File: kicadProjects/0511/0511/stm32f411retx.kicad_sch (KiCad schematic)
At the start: 9 parts, among them U8 STM32F411RETx

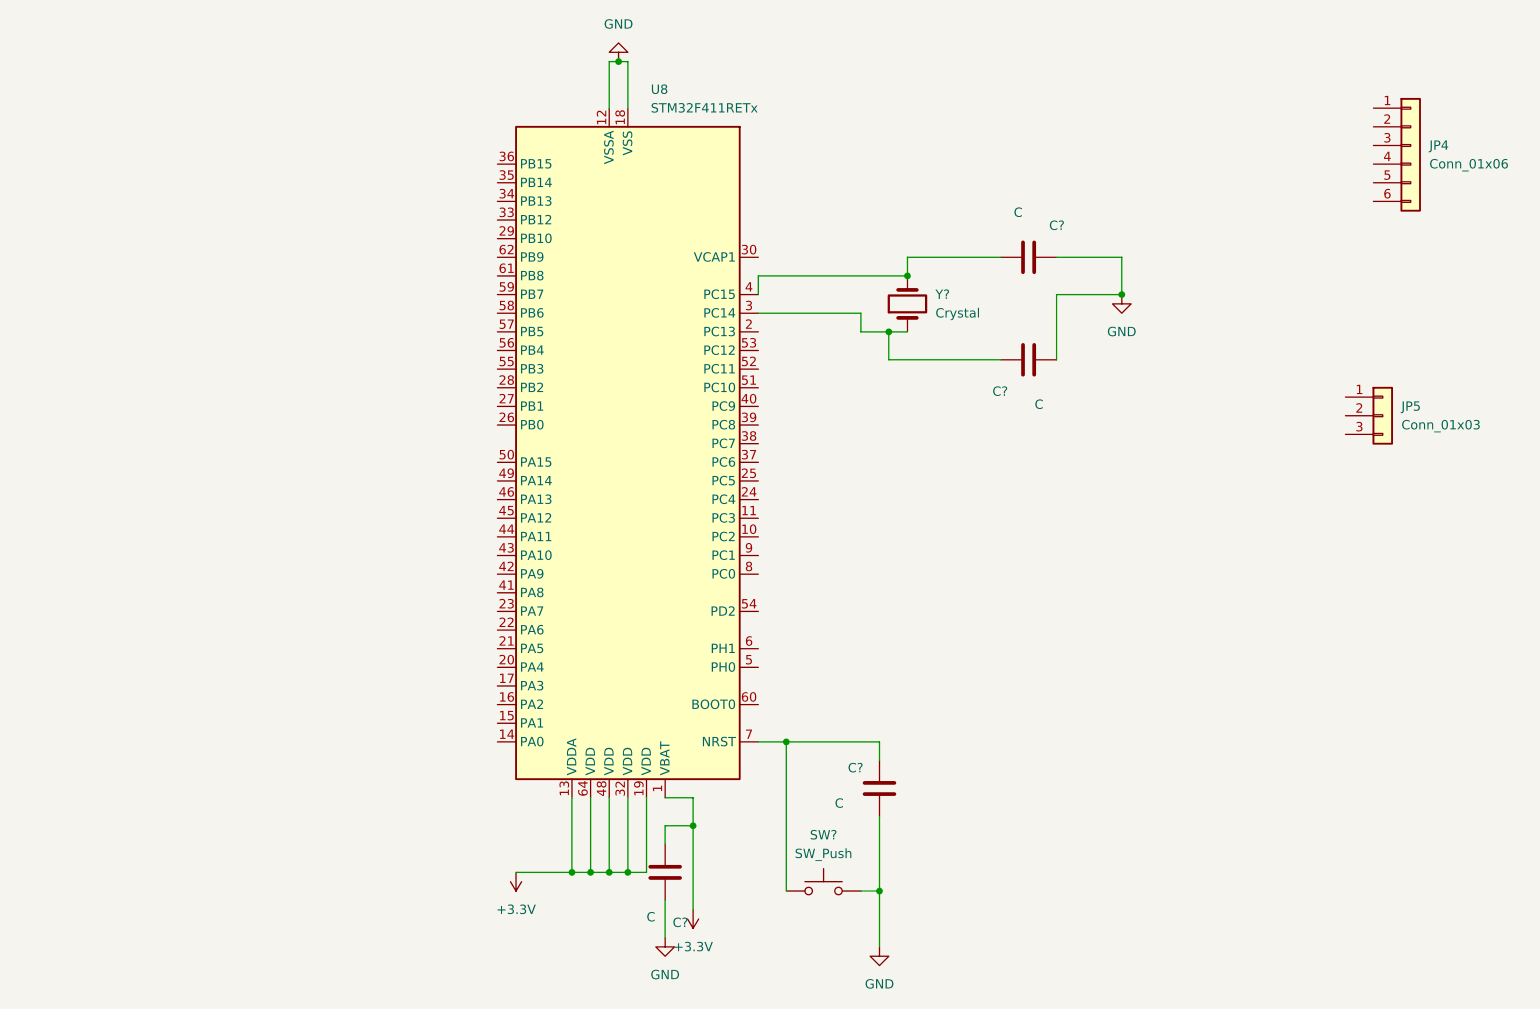
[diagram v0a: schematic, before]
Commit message: stm32 bloc implementation
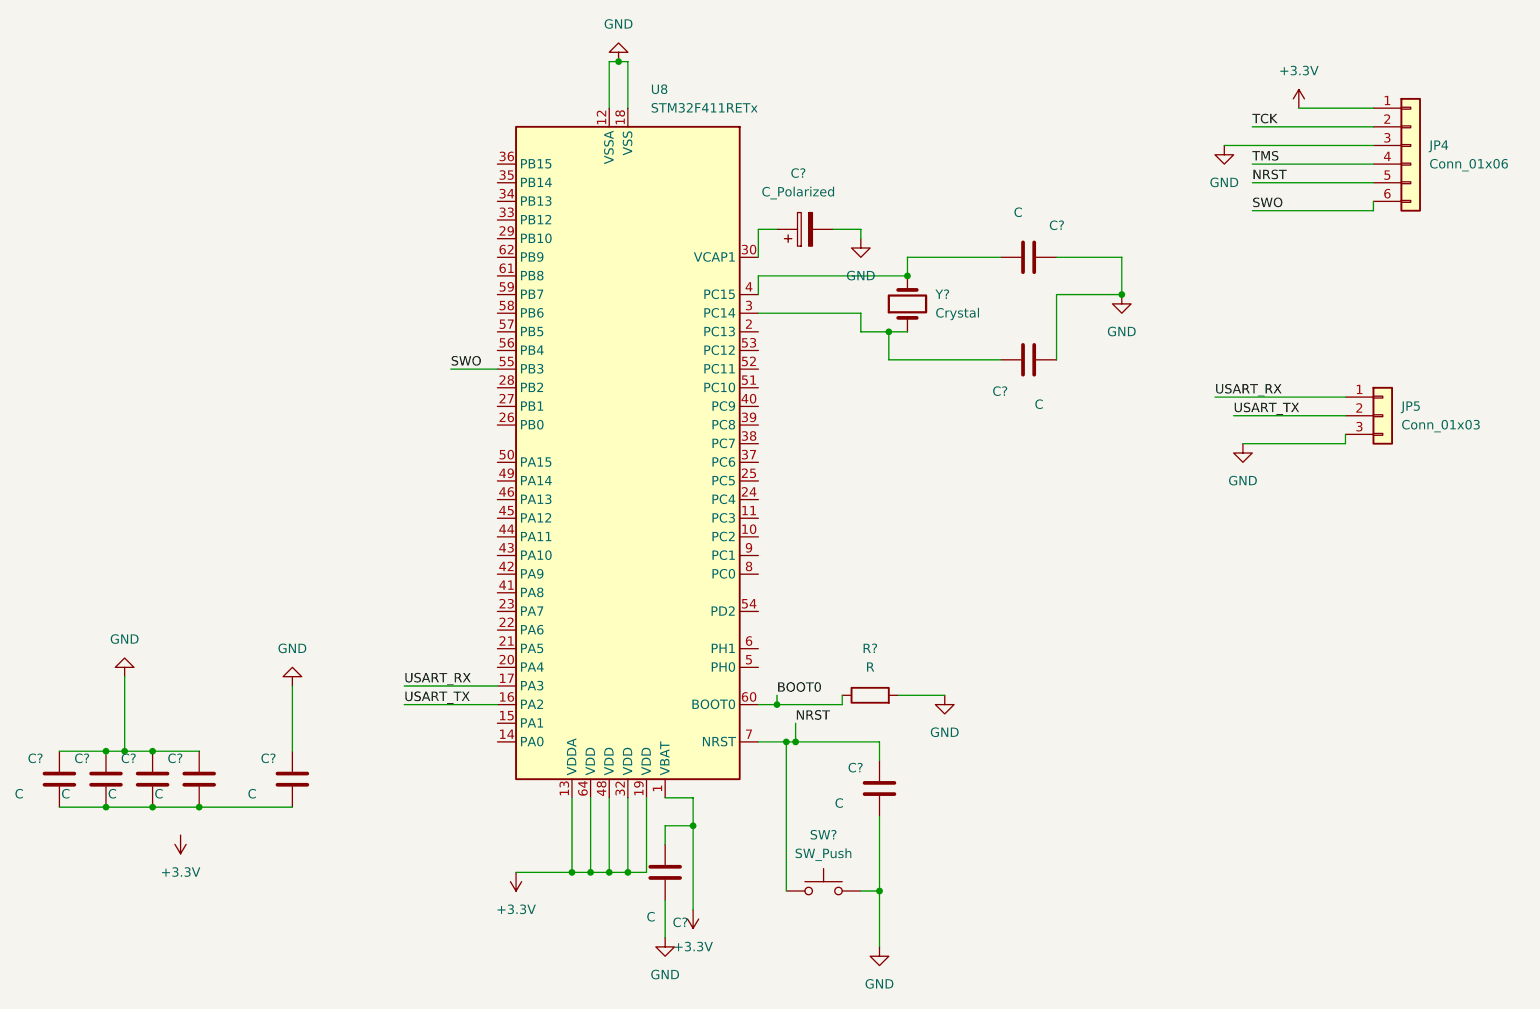
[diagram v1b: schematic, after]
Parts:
- added C? (x5): C, symbol Device:C
- added C?: C_Polarized, symbol Device:C_Polarized
- added R?: R, symbol Device:R
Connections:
- net +3.3V: now also JP4.1 (Pin_1)
- net GND: now also JP4.3 (Pin_3), JP5.3 (Pin_3), C?.1, C?.1, C?.1, C?.1, C?.1, C?.2, R?.2
- net USART_TX: now reaches U8.16 (PA2)
- net USART_TX: now also JP5.2 (Pin_2)
- net USART_RX: now reaches U8.17 (PA3)
- net USART_RX: now also JP5.1 (Pin_1)
- net at U8.30 (VCAP1): now also C?.1
- net SWO: now reaches U8.55 (PB3)
- net SWO: now also JP4.6 (Pin_6)
- net BOOT0: now reaches U8.60 (BOOT0)
- net BOOT0: now also R?.1
- net NRST: now reaches C?.1, SW?.1, U8.7 (NRST)
- net NRST: now also JP4.5 (Pin_5)
- net TCK: now reaches JP4.2 (Pin_2)
- net TMS: now reaches JP4.4 (Pin_4)
- new net: C?.2, C?.2, C?.2, C?.2, C?.2
